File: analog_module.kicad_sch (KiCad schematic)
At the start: 25 parts, among them J20 Conn_01x02_Female, J24 Conn_01x02_Female, J25 Conn_01x02_Female, J26 Conn_01x02_Female, SW12 SW_SPST, SW13 SW_SPST, SW14 SW_SPST, SW15 SW_SPST, U42 ADS1115

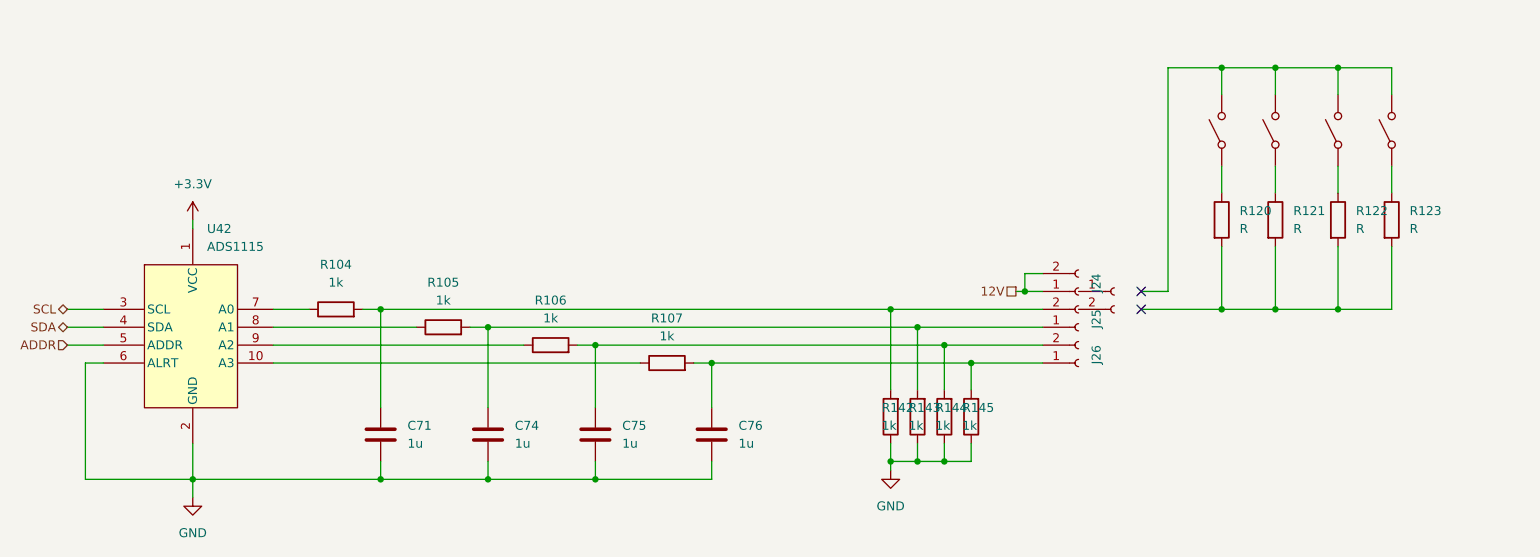
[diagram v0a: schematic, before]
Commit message: v2.1 finished
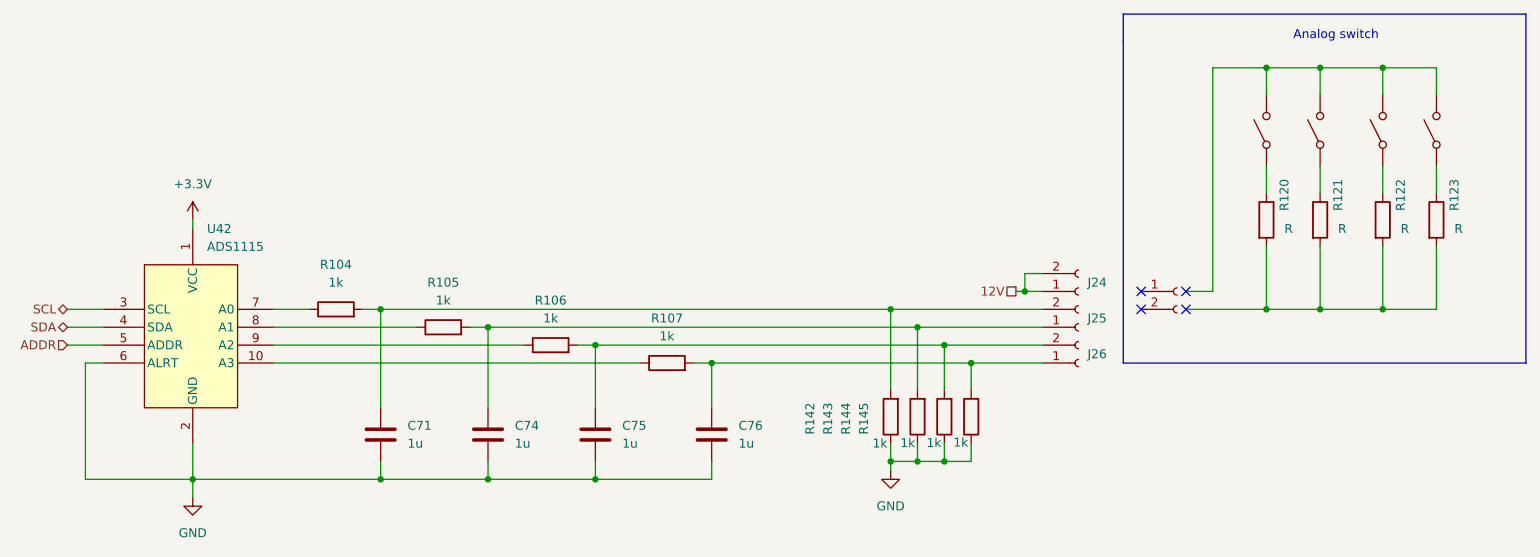
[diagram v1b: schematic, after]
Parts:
- R142, R143, R144, R145: footprint Resistor_THT:R_Axial_DIN0204_L3.6mm_D1.6mm_P7.62mm_Horizontal -> Resistor_SMD:R_0805_2012Metric_Pad1.20x1.40mm_HandSolder
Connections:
- no-connect marks 2 -> 4
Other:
- note added: "Analog switch"
- moved on the sheet: R120, R121, R122, R123
